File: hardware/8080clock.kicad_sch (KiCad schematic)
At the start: 0 parts

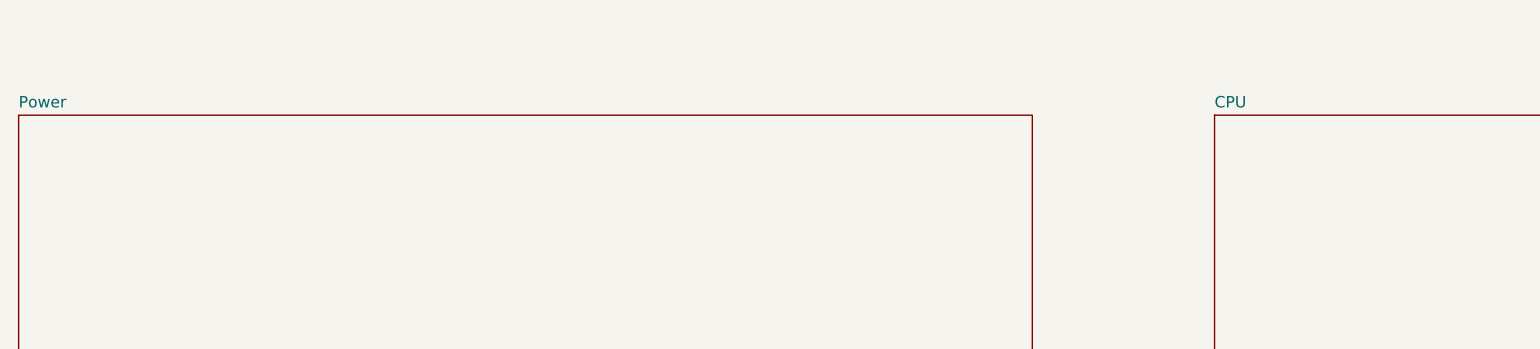
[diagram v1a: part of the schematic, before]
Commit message: Update 25.05.2026
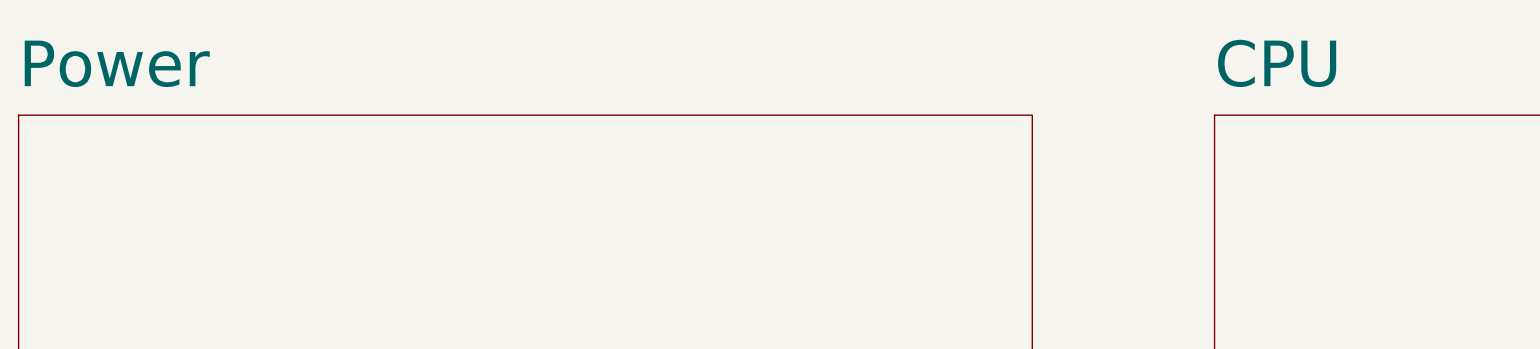
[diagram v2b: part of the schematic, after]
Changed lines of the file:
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@@
 		)
 		(property "Sheetname" "CPU"
-			(at 160.02 32.3084 0)
+			(at 160.02 30.4034 0)
 			(show_name no)
 			(do_not_autoplace no)
 			(effects
 				(font
-					(size 1.27 1.27)
+					(size 5.08 5.08)
 				)
 				(justify left bottom)
@@
 		)
 		(property "Sheetname" "Power"
-			(at 26.67 32.3084 0)
+			(at 26.67 30.4034 0)
 			(show_name no)
 			(do_not_autoplace no)
 			(effects
 				(font
-					(size 1.27 1.27)
+					(size 5.08 5.08)
 				)
 				(justify left bottom)
